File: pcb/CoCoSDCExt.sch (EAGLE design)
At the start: 48 parts, among them IC1 AM29F040J, IC10 YAC512-M, IC14 TL974, IC15 TL974, IC2 XC9572XLVQG64, IC9 YMF262-M, X1 EXPANSION_PORT_COCO, X2 EXPANSION_PORT_COCOS

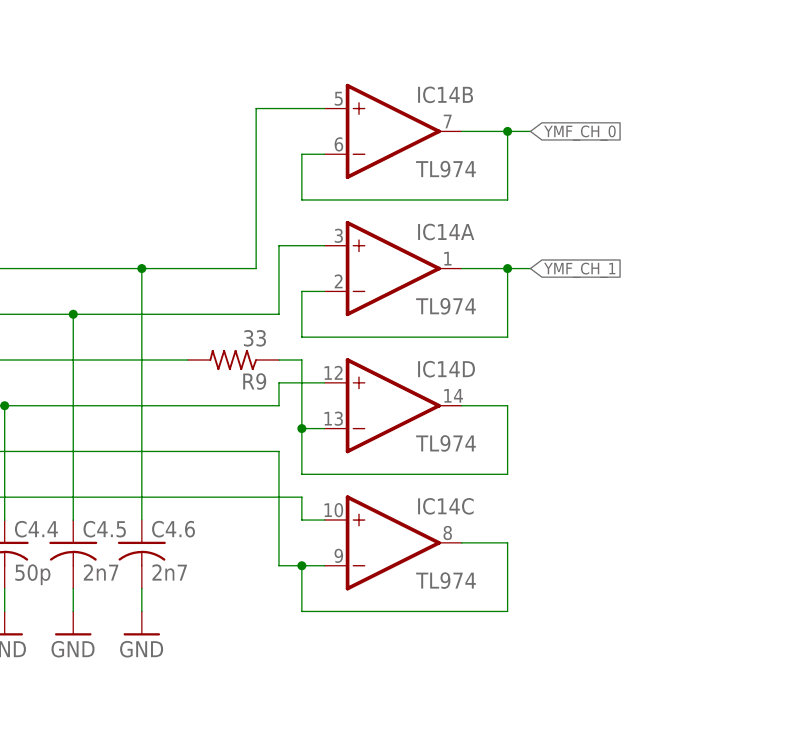
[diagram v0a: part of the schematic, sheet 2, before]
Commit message: positioning
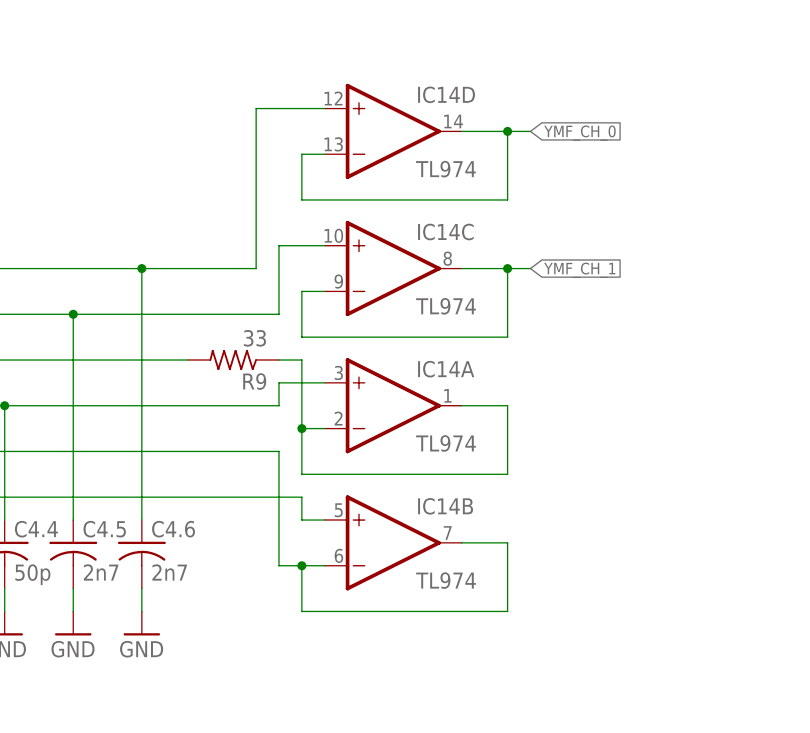
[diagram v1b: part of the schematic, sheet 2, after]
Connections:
- net N$18: now also IC14A.-IN, IC14A.OUT; no longer IC14D.-IN, IC14D.OUT
- net N$19: now also IC14D.+IN; no longer IC14B.+IN
- net N$20: now also IC14C.+IN; no longer IC14A.+IN
- net N$23: now also IC14A.+IN; no longer IC14D.+IN
- net N$26: now also IC14B.-IN, IC14B.OUT; no longer IC14C.-IN, IC14C.OUT
- net N$28: now also IC14B.+IN; no longer IC14C.+IN
- net YMF_CH_0: now also IC14D.-IN, IC14D.OUT; no longer IC14B.-IN, IC14B.OUT
- net YMF_CH_1: now also IC14C.-IN, IC14C.OUT; no longer IC14A.-IN, IC14A.OUT
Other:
- moved on the sheet: IC14A, IC14B, IC14C, IC14D
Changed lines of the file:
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@@
 <instance part="C19" gate="G$1" x="134.62" y="58.42" rot="R90"/>
 <instance part="C20" gate="G$1" x="220.98" y="68.58" rot="R90"/>
-<instance part="IC14" gate="A" x="203.2" y="182.88"/>
-<instance part="IC14" gate="B" x="203.2" y="198.12"/>
-<instance part="IC14" gate="C" x="203.2" y="152.4"/>
-<instance part="IC14" gate="D" x="203.2" y="167.64"/>
+<instance part="IC14" gate="C" x="203.2" y="182.88"/>
+<instance part="IC14" gate="D" x="203.2" y="198.12"/>
+<instance part="IC14" gate="B" x="203.2" y="152.4"/>
+<instance part="IC14" gate="A" x="203.2" y="167.64"/>
 <instance part="IC15" gate="A" x="185.42" y="78.74"/>
 <instance part="IC15" gate="B" x="205.74" y="68.58"/>
@@
 <wire x1="175.26" y1="154.94" x2="175.26" y2="182.88" width="0.1524" layer="91"/>
 <junction x="175.26" y="182.88"/>
-<pinref part="IC14" gate="B" pin="+IN"/>
+<pinref part="IC14" gate="D" pin="+IN"/>
 </segment>
 </net>
@@
 <wire x1="167.64" y1="154.94" x2="167.64" y2="177.8" width="0.1524" layer="91"/>
 <junction x="167.64" y="177.8"/>
-<pinref part="IC14" gate="A" pin="+IN"/>
+<pinref part="IC14" gate="C" pin="+IN"/>
 </segment>
 </net>
@@
 <junction x="215.9" y="182.88"/>
 <label x="218.44" y="182.88" size="1.27" layer="95" xref="yes"/>
-<pinref part="IC14" gate="A" pin="-IN"/>
-<pinref part="IC14" gate="A" pin="OUT"/>
+<pinref part="IC14" gate="C" pin="-IN"/>
+<pinref part="IC14" gate="C" pin="OUT"/>
 </segment>
 <segment>
@@
 <wire x1="215.9" y1="160.02" x2="215.9" y2="167.64" width="0.1524" layer="91"/>
 <wire x1="215.9" y1="167.64" x2="210.82" y2="167.64" width="0.1524" layer="91"/>
-<pinref part="IC14" gate="D" pin="-IN"/>
-<pinref part="IC14" gate="D" pin="OUT"/>
+<pinref part="IC14" gate="A" pin="-IN"/>
+<pinref part="IC14" gate="A" pin="OUT"/>
 </segment>
 </net>
@@
 <wire x1="160.02" y1="167.64" x2="190.5" y2="167.64" width="0.1524" layer="91"/>
 <wire x1="190.5" y1="167.64" x2="190.5" y2="170.18" width="0.1524" layer="91"/>
-<pinref part="IC14" gate="D" pin="+IN"/>
+<pinref part="IC14" gate="A" pin="+IN"/>
 </segment>
 </net>
@@
 <wire x1="190.5" y1="149.86" x2="193.04" y2="149.86" width="0.1524" layer="91"/>
 <junction x="193.04" y="149.86"/>
-<pinref part="IC14" gate="C" pin="-IN"/>
-<pinref part="IC14" gate="C" pin="OUT"/>
+<pinref part="IC14" gate="B" pin="-IN"/>
+<pinref part="IC14" gate="B" pin="OUT"/>
 </segment>
 </net>
@@
 <junction x="152.4" y="157.48"/>
 <pinref part="C4.2" gate="G$1" pin="1"/>
-<pinref part="IC14" gate="C" pin="+IN"/>
+<pinref part="IC14" gate="B" pin="+IN"/>
 </segment>
 </net>
@@
 <junction x="215.9" y="198.12"/>
 <label x="218.44" y="198.12" size="1.27" layer="95" xref="yes"/>
-<pinref part="IC14" gate="B" pin="-IN"/>
-<pinref part="IC14" gate="B" pin="OUT"/>
-</segment>
-<segment>
+<pinref part="IC14" gate="D" pin="-IN"/>
+<pinref part="IC14" gate="D" pin="OUT"/>
+</segment>
+<segment>
